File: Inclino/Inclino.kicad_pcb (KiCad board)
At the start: 2 copper layers, 171.4 x 91.4 mm, 44 parts, among them P1 Prog, Q1 PMV65UN, SW1 SW_Push, SW2 SW_Push, SW3 SW_Push, SW4 SW_Push, U1 MAX7219, U10 TPS61032PWP, U2 SCA103T-D04, U3 7SEGMENT_CC, U4 7SEGMENT_CC, U5 7SEGMENT_CC, U6 7SEGMENT_CC, U7 PIC16F18323_SOIC, U8 7SEGMENT_CC, U9 7SEGMENT_CC

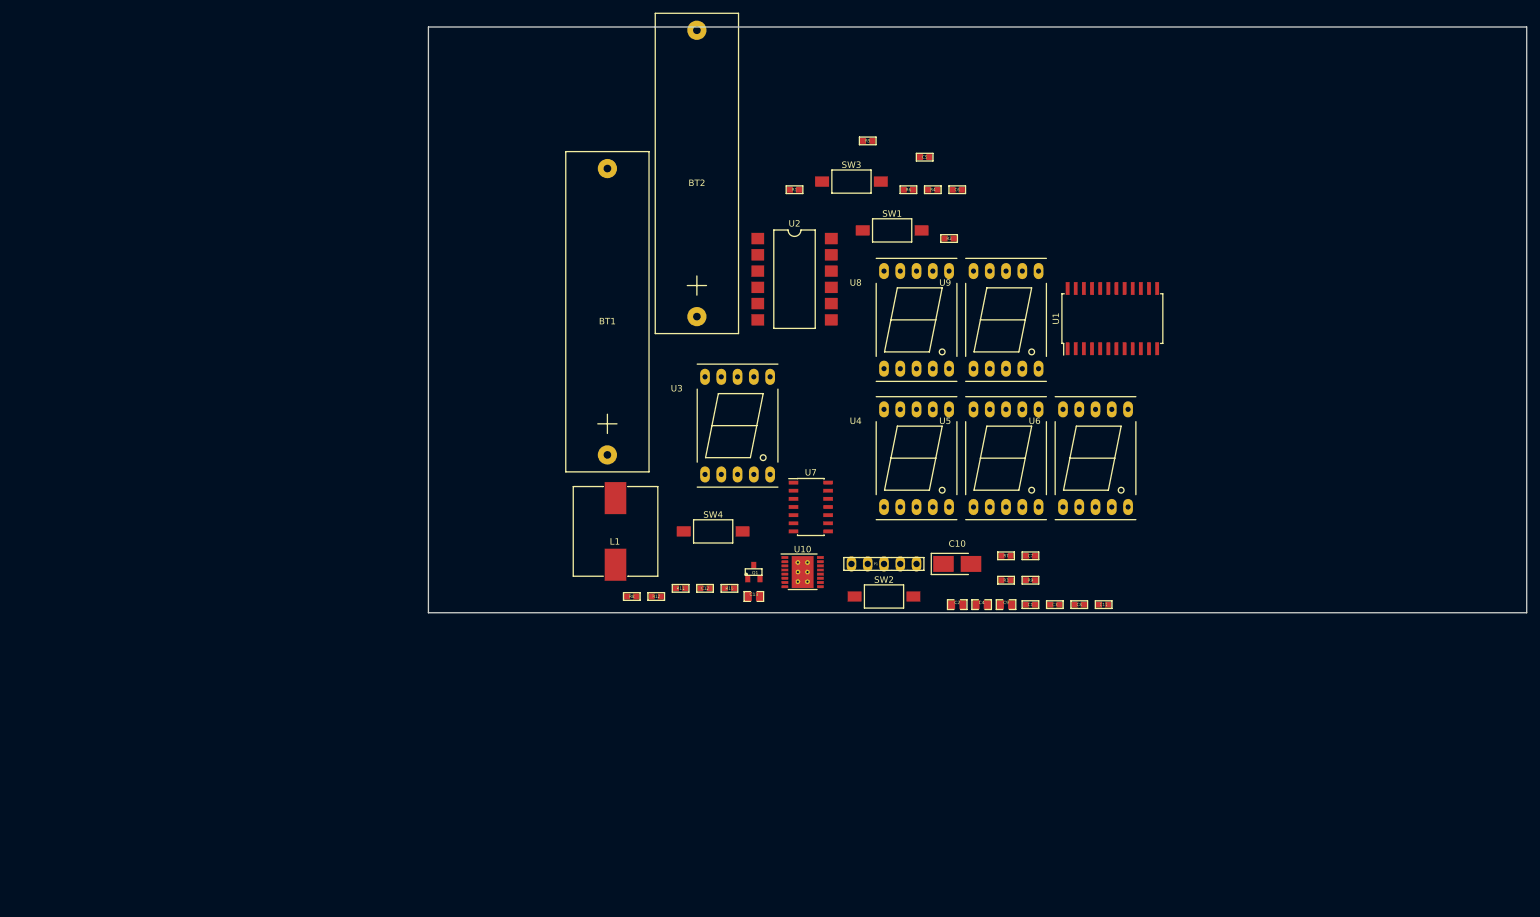
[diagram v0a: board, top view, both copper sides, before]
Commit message: Send Inclino PCB
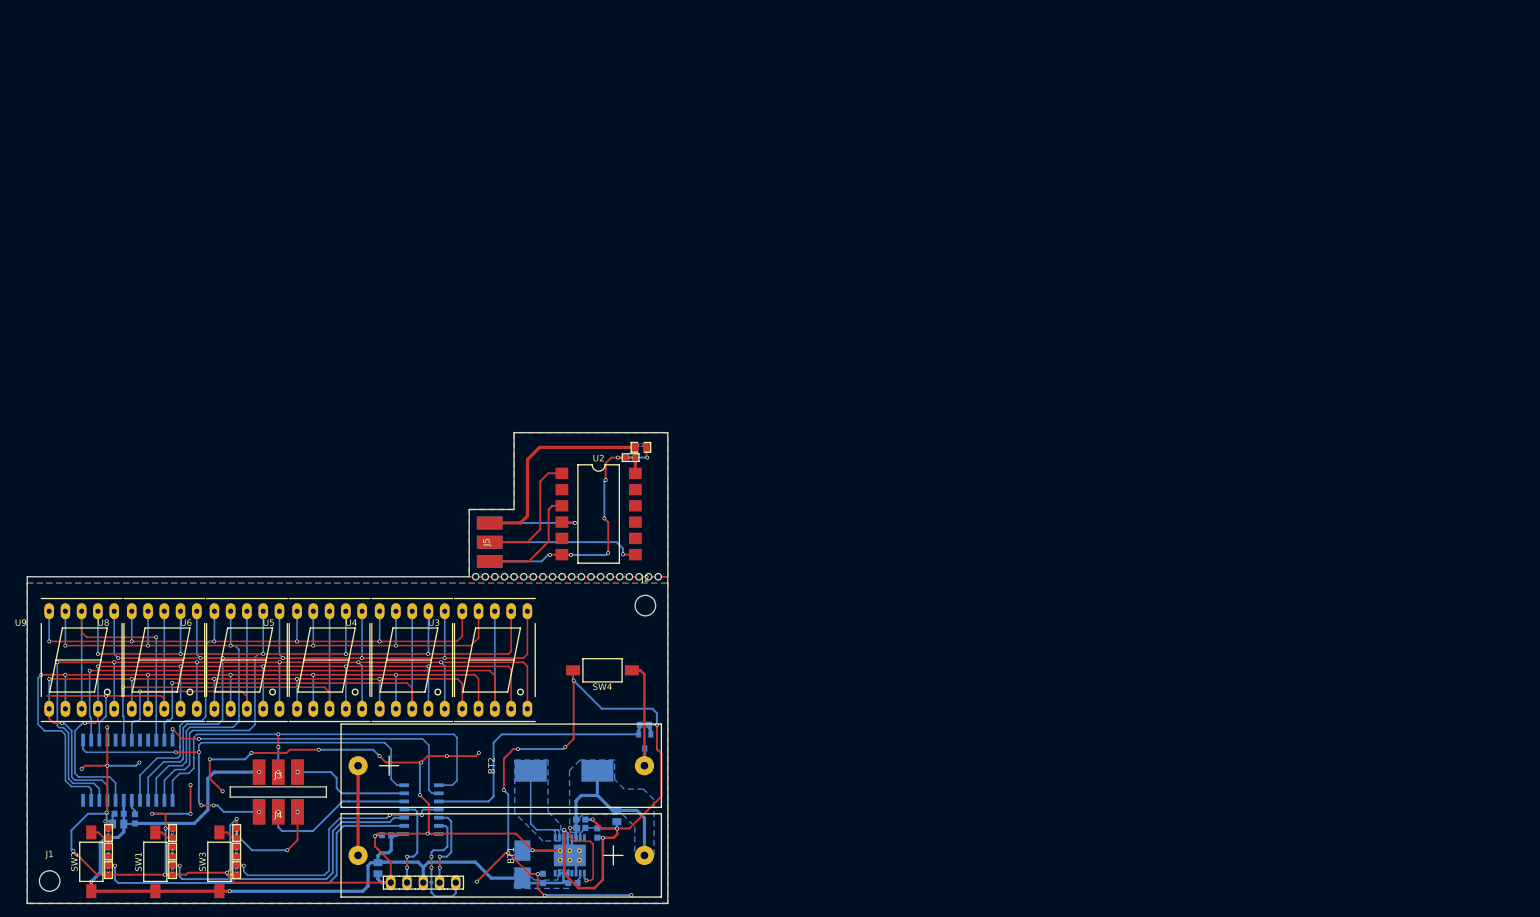
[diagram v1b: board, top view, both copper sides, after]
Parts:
- removed R8: 100k, Yame_library:SM0603-MR
- added CutHole_1: VAL**, Yame_library:CutHole_1, F.Cu at (110.0, 129.0)
- added CutHole_1: VAL**, Yame_library:CutHole_1, F.Cu at (122.0, 129.0)
- added CutHole_1: VAL**, Yame_library:CutHole_1, F.Cu at (107.0, 129.0)
- added CutHole_1: VAL**, Yame_library:CutHole_1, F.Cu at (108.5, 129.0)
- added CutHole_1: VAL**, Yame_library:CutHole_1, F.Cu at (105.5, 129.0)
- added CutHole_1: VAL**, Yame_library:CutHole_1, F.Cu at (95.0, 129.0)
- added CutHole_1: VAL**, Yame_library:CutHole_1, F.Cu at (98.0, 129.0)
- added CutHole_1: VAL**, Yame_library:CutHole_1, F.Cu at (96.5, 129.0)
- added CutHole_1: VAL**, Yame_library:CutHole_1, F.Cu at (102.5, 129.0)
- added CutHole_1: VAL**, Yame_library:CutHole_1, F.Cu at (104.0, 129.0)
- added CutHole_1: VAL**, Yame_library:CutHole_1, F.Cu at (101.0, 129.0)
- added CutHole_1: VAL**, Yame_library:CutHole_1, F.Cu at (111.5, 129.0)
- added CutHole_1: VAL**, Yame_library:CutHole_1, F.Cu at (99.5, 129.0)
- added CutHole_1: VAL**, Yame_library:CutHole_1, F.Cu at (114.5, 129.0)
- added CutHole_1: VAL**, Yame_library:CutHole_1, F.Cu at (113.0, 129.0)
- added CutHole_1: VAL**, Yame_library:CutHole_1, F.Cu at (119.0, 129.0)
- added CutHole_1: VAL**, Yame_library:CutHole_1, F.Cu at (120.5, 129.0)
- added CutHole_1: VAL**, Yame_library:CutHole_1, F.Cu at (117.5, 129.0)
- added CutHole_1: VAL**, Yame_library:CutHole_1, F.Cu at (116.0, 129.0)
- added CutHole_1: VAL**, Yame_library:CutHole_1, F.Cu at (123.5, 129.0)
- added J1: Fix, Mounting_Holes:MountingHole_3.2mm_M3, F.Cu at (28.5, 176.5)
- added J2: Fix, Mounting_Holes:MountingHole_3.2mm_M3, F.Cu at (121.5, 133.5)
- added J3: Conn_01x03, Yame_library:Inc_90°, F.Cu at (64.2, 159.5)
- added J4: Conn_01x03, Yame_library:Inc_90°, F.Cu at (64.2, 165.7)
- added J5: Conn_01x03, Yame_library:Inc_90°, F.Cu at (97.2, 123.6)
- added J6: Conn_01x03, Yame_library:Inc_90°, B.Cu at (97.2, 123.6)
- C10, C11, C12, C13, C3, C4, C8, C9, L1, Q1, R1, R10, R11, R12, R9, U1, U10, U7: moved to B.Cu
- SW4: value SW_Push -> SW_Power
- moved U1 169.1 mm to (40.7, 159.2), turned to 270 degrees
- moved C6 162.1 mm to (47.7, 174.8), turned to 270 degrees
- moved C5 154.7 mm to (57.7, 174.8), turned to 270 degrees
- moved R6 154.5 mm to (47.7, 171.9), turned to 90 degrees
- moved U9 153.8 mm to (33.5, 142.0)
- moved R2 152.7 mm to (47.7, 169.0), turned to 90 degrees
- moved C7 152.0 mm to (37.7, 174.8), turned to 270 degrees
- moved SW1 151.5 mm to (45.0, 173.5), turned to 90 degrees
- moved C3 149.7 mm to (39.4, 166.0), turned to 180 degrees
- moved R5 148.4 mm to (57.7, 171.9), turned to 90 degrees
- moved R4 148.0 mm to (57.7, 169.0), turned to 90 degrees
- moved R7 147.5 mm to (37.7, 171.9), turned to 90 degrees
- moved R3 145.6 mm to (37.7, 169.0), turned to 90 degrees
- moved SW3 145.0 mm to (55.0, 173.5), turned to 90 degrees
- moved R1 142.3 mm to (41.8, 166.8), turned to 90 degrees
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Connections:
- net Net-(L1-Pad2) renamed /+Vsw
- BT2 pad 2: Net-(BT2-Pad2) -> /BATT_LowSide
- C1 pad 1: /+5v -> /+5v_R
- C1 pad 2: GND -> /GND_R
- C2 pad 1: /+5v -> /+5v_R
- C2 pad 2: GND -> /GND_R
- Q1 pad 2: Net-(BT2-Pad2) -> GND
- Q1 pad 3: GND -> /BATT_LowSide
- R12 pad 1: Net-(BT2-Pad2) -> /Von
- R12 pad 2: /Von -> GND
- SW4 pad 1: /+Vbat -> /BATT_LowSide
- SW4 pad 2: /Von -> GND
- U2 pad 1: /SCK -> /SCK_R
- U2 pad 12: /+5v -> /+5v_R
- U2 pad 3: /MISO -> /MISO_R
- U2 pad 4: /MOSI -> /MOSI_R
- U2 pad 6: GND -> /GND_R
- U2 pad 7: //CS_INC -> //CS_INC_R
- U7 pad 10: Net-(R8-Pad2) -> /Von
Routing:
- net GND: track 0.00 -> 412.6 mm, vias 0 -> 42
- net /DP: track 0.00 -> 143.7 mm, vias 0 -> 6
- net /A: track 0.00 -> 140.1 mm, vias 0 -> 5
- net /B: track 0.00 -> 139.6 mm, vias 0 -> 6
- net /+5v: track 0.00 -> 138.7 mm, vias 0 -> 3
- net /F: track 0.00 -> 131.7 mm, vias 0 -> 5
- net /C: track 0.00 -> 126.4 mm, vias 0 -> 6
- net /D: track 0.00 -> 126.2 mm, vias 0 -> 6
- net /G: track 0.00 -> 125.8 mm, vias 0 -> 5
- net /E: track 0.00 -> 113.6 mm, vias 0 -> 6
- net /D0: track 0.00 -> 94.9 mm, vias 0 -> 1
- net /MOSI: track 0.00 -> 76.4 mm, vias 0 -> 5
- net /SCK: track 0.00 -> 69.3 mm, vias 0 -> 3
- net /D1: track 0.00 -> 65.9 mm, vias 0 -> 1
- net /D2: track 0.00 -> 58.7 mm, vias 0 -> 1
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- added copper zone on B.Cu, net /+5v
- added copper zone on B.Cu, net /+Vbat
- added copper zone on B.Cu, net /+Vsw
- added copper zone on B.Cu, net /GND_R
- added copper zone on F.Cu, net /GND_R
- added copper zone on B.Cu, net GND
- added copper zone on F.Cu, net GND
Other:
- board size 171.4 x 91.4 mm -> 100 x 73.5 mm
